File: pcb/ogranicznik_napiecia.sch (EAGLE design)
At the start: 6 parts, among them T1 BD235

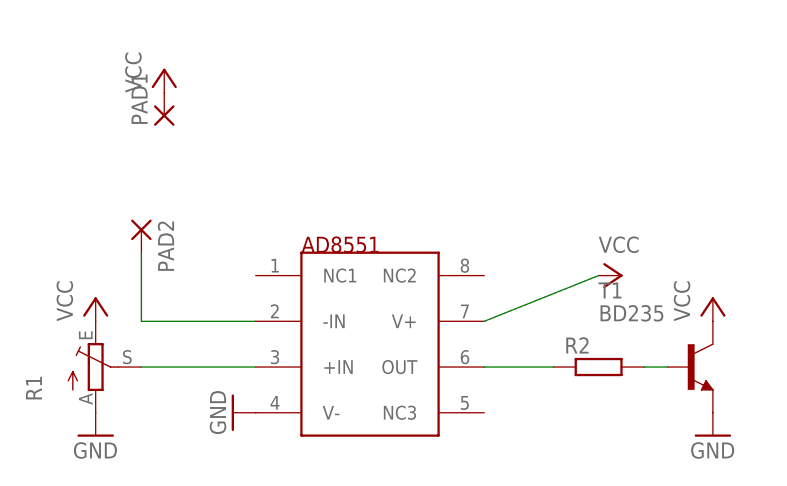
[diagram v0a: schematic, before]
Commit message: fuel gauge tutorial, mgr update
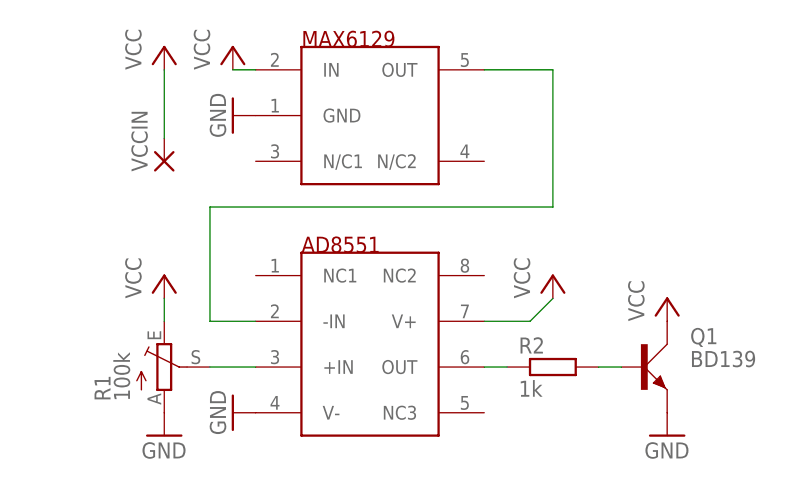
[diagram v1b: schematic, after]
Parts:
- removed PAD1, PAD2: (no value), wirepad:2,54/0,9
- removed T1: BD235, transistor:BD235
- added Q1: BD139, transistor-power:BD139
- added U$2: MAX6129, ref-packages:MAX6129
- added VCCIN: (no value), wirepad:2,54/0,9
- R1: value (none) -> 100k
- R2: value (none) -> 1k
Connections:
- net GND: now also Q1.E, U$2.GND; no longer T1.E
- net N$1: now also Q1.B; no longer T1.B
- net N$4: now also U$2.OUT; no longer PAD2.P
- net VCC: now also Q1.C, U$2.IN, VCCIN.P; no longer PAD1.P, T1.C
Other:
- moved on the sheet: R1, R2
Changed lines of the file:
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@@
 <parts>
 <part name="U$1" library="ref-packages" deviceset="AD8551" device=""/>
-<part name="R1" library="pot" deviceset="TRIM_EU-" device="RJ9W"/>
+<part name="R1" library="pot" deviceset="TRIM_EU-" device="RJ9W" value="100k"/>
 <part name="GND1" library="supply1" deviceset="GND" device=""/>
 <part name="GND2" library="supply1" deviceset="GND" device=""/>
-<part name="T1" library="transistor" deviceset="BD235" device=""/>
-<part name="R2" library="rcl" deviceset="R-EU_" device="M0805"/>
+<part name="R2" library="rcl" deviceset="R-EU_" device="M0805" value="1k"/>
 <part name="GND3" library="supply1" deviceset="GND" device=""/>
 <part name="P+1" library="supply1" deviceset="VCC" device=""/>
@@
 <part name="P+3" library="supply1" deviceset="VCC" device=""/>
 <part name="P+4" library="supply1" deviceset="VCC" device=""/>
-<part name="PAD1" library="wirepad" deviceset="2,54/0,9" device=""/>
-<part name="PAD2" library="wirepad" deviceset="2,54/0,9" device=""/>
+<part name="VCCIN" library="wirepad" deviceset="2,54/0,9" device=""/>
+<part name="U$2" library="ref-packages" deviceset="MAX6129" device=""/>
+<part name="P+5" library="supply1" deviceset="VCC" device=""/>
+<part name="GND4" library="supply1" deviceset="GND" device=""/>
+<part name="Q1" library="transistor-power" deviceset="BD139" device=""/>
 </parts>
 <sheets>
@@
 <instances>
 <instance part="U$1" gate="G$1" x="63.5" y="43.18"/>
-<instance part="R1" gate="1" x="33.02" y="40.64"/>
-<instance part="GND1" gate="1" x="33.02" y="33.02"/>
+<instance part="R1" gate="1" x="40.64" y="40.64"/>
+<instance part="GND1" gate="1" x="40.64" y="33.02"/>
 <instance part="GND2" gate="1" x="48.26" y="35.56" rot="R270"/>
-<instance part="T1" gate="G$1" x="99.06" y="40.64"/>
-<instance part="R2" gate="G$1" x="88.9" y="40.64"/>
-<instance part="GND3" gate="1" x="101.6" y="33.02"/>
-<instance part="P+1" gate="VCC" x="33.02" y="48.26"/>
-<instance part="P+2" gate="VCC" x="101.6" y="48.26"/>
-<instance part="P+3" gate="VCC" x="91.44" y="50.8" rot="R270"/>
-<instance part="P+4" gate="VCC" x="40.64" y="73.66"/>
-<instance part="PAD1" gate="1" x="40.64" y="68.58" rot="R90"/>
-<instance part="PAD2" gate="1" x="38.1" y="55.88" rot="R270"/>
+<instance part="R2" gate="G$1" x="83.82" y="40.64"/>
+<instance part="GND3" gate="1" x="96.52" y="33.02"/>
+<instance part="P+1" gate="VCC" x="40.64" y="50.8"/>
+<instance part="P+2" gate="VCC" x="96.52" y="48.26"/>
+<instance part="P+3" gate="VCC" x="83.82" y="50.8"/>
+<instance part="P+4" gate="VCC" x="40.64" y="76.2"/>
+<instance part="VCCIN" gate="1" x="40.64" y="63.5" rot="R90"/>
+<instance part="U$2" gate="G$1" x="63.5" y="68.58"/>
+<instance part="P+5" gate="VCC" x="48.26" y="76.2"/>
+<instance part="GND4" gate="1" x="48.26" y="68.58" rot="R270"/>
+<instance part="Q1" gate="1" x="93.98" y="40.64"/>
 </instances>
 <busses>
@@
 </segment>
 <segment>
-<pinref part="T1" gate="G$1" pin="E"/>
+<pinref part="U$2" gate="G$1" pin="GND"/>
+<pinref part="GND4" gate="1" pin="GND"/>
+</segment>
+<segment>
 <pinref part="GND3" gate="1" pin="GND"/>
+<pinref part="Q1" gate="1" pin="E"/>
 </segment>
 </net>
 <net name="N$1" class="0">
 <segment>
-<pinref part="T1" gate="G$1" pin="B"/>
 <pinref part="R2" gate="G$1" pin="2"/>
-<wire x1="96.52" y1="40.64" x2="93.98" y2="40.64" width="0.1524" layer="91"/>
+<wire x1="91.44" y1="40.64" x2="88.9" y2="40.64" width="0.1524" layer="91"/>
+<pinref part="Q1" gate="1" pin="B"/>
 </segment>
 </net>
@@
 <pinref part="R2" gate="G$1" pin="1"/>
 <pinref part="U$1" gate="G$1" pin="OUT"/>
-<wire x1="83.82" y1="40.64" x2="76.2" y2="40.64" width="0.1524" layer="91"/>
+<wire x1="78.74" y1="40.64" x2="76.2" y2="40.64" width="0.1524" layer="91"/>
 </segment>
 </net>
@@
 <pinref part="R1" gate="1" pin="E"/>
 <pinref part="P+1" gate="VCC" pin="VCC"/>
-</segment>
-<segment>
-<pinref part="T1" gate="G$1" pin="C"/>
-<pinref part="P+2" gate="VCC" pin="VCC"/>
+<wire x1="40.64" y1="45.72" x2="40.64" y2="48.26" width="0.1524" layer="91"/>
 </segment>
 <segment>
 <pinref part="U$1" gate="G$1" pin="V+"/>
 <pinref part="P+3" gate="VCC" pin="VCC"/>
-<wire x1="88.9" y1="50.8" x2="76.2" y2="45.72" width="0.1524" layer="91"/>
+<wire x1="83.82" y1="48.26" x2="81.28" y2="45.72" width="0.1524" layer="91"/>
+<wire x1="81.28" y1="45.72" x2="76.2" y2="45.72" width="0.1524" layer="91"/>
 </segment>
 <segment>
 <pinref part="P+4" gate="VCC" pin="VCC"/>
-<pinref part="PAD1" gate="1" pin="P"/>
+<pinref part="VCCIN" gate="1" pin="P"/>
+<wire x1="40.64" y1="73.66" x2="40.64" y2="66.04" width="0.1524" layer="91"/>
+</segment>
+<segment>
+<pinref part="U$2" gate="G$1" pin="IN"/>
+<pinref part="P+5" gate="VCC" pin="VCC"/>
+<wire x1="48.26" y1="73.66" x2="50.8" y2="73.66" width="0.1524" layer="91"/>
+</segment>
+<segment>
+<pinref part="P+2" gate="VCC" pin="VCC"/>
+<pinref part="Q1" gate="1" pin="C"/>
 </segment>
 </net>
@@
 <pinref part="R1" gate="1" pin="S"/>
 <pinref part="U$1" gate="G$1" pin="+IN"/>
-<wire x1="38.1" y1="40.64" x2="50.8" y2="40.64" width="0.1524" layer="91"/>
+<wire x1="45.72" y1="40.64" x2="50.8" y2="40.64" width="0.1524" layer="91"/>
 </segment>
 </net>
@@
 <segment>
 <pinref part="U$1" gate="G$1" pin="-IN"/>
-<pinref part="PAD2" gate="1" pin="P"/>
-<wire x1="38.1" y1="53.34" x2="38.1" y2="45.72" width="0.1524" layer="91"/>
-<wire x1="38.1" y1="45.72" x2="50.8" y2="45.72" width="0.1524" layer="91"/>
+<wire x1="45.72" y1="58.42" x2="45.72" y2="45.72" width="0.1524" layer="91"/>
+<wire x1="45.72" y1="45.72" x2="50.8" y2="45.72" width="0.1524" layer="91"/>
+<wire x1="45.72" y1="58.42" x2="83.82" y2="58.42" width="0.1524" layer="91"/>
+<wire x1="83.82" y1="58.42" x2="83.82" y2="73.66" width="0.1524" layer="91"/>
+<pinref part="U$2" gate="G$1" pin="OUT"/>
+<wire x1="83.82" y1="73.66" x2="76.2" y2="73.66" width="0.1524" layer="91"/>
 </segment>
 </net>
